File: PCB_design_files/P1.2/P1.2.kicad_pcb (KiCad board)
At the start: 2 copper layers, 127 x 127 mm, 37 parts, among them J1 -EEG_INPUT, J2 +EEG_INPUT, J3 +3.3V, J4 GND, J5 -3V3, J6 EEG_INPUT, J7 STAGE_1_OUT, J8 STAGE_2_OUT, J9 STAGE_3_OUT, U1 INA819, U2 TPS61094, U3 TLV9102, U4 TC1044

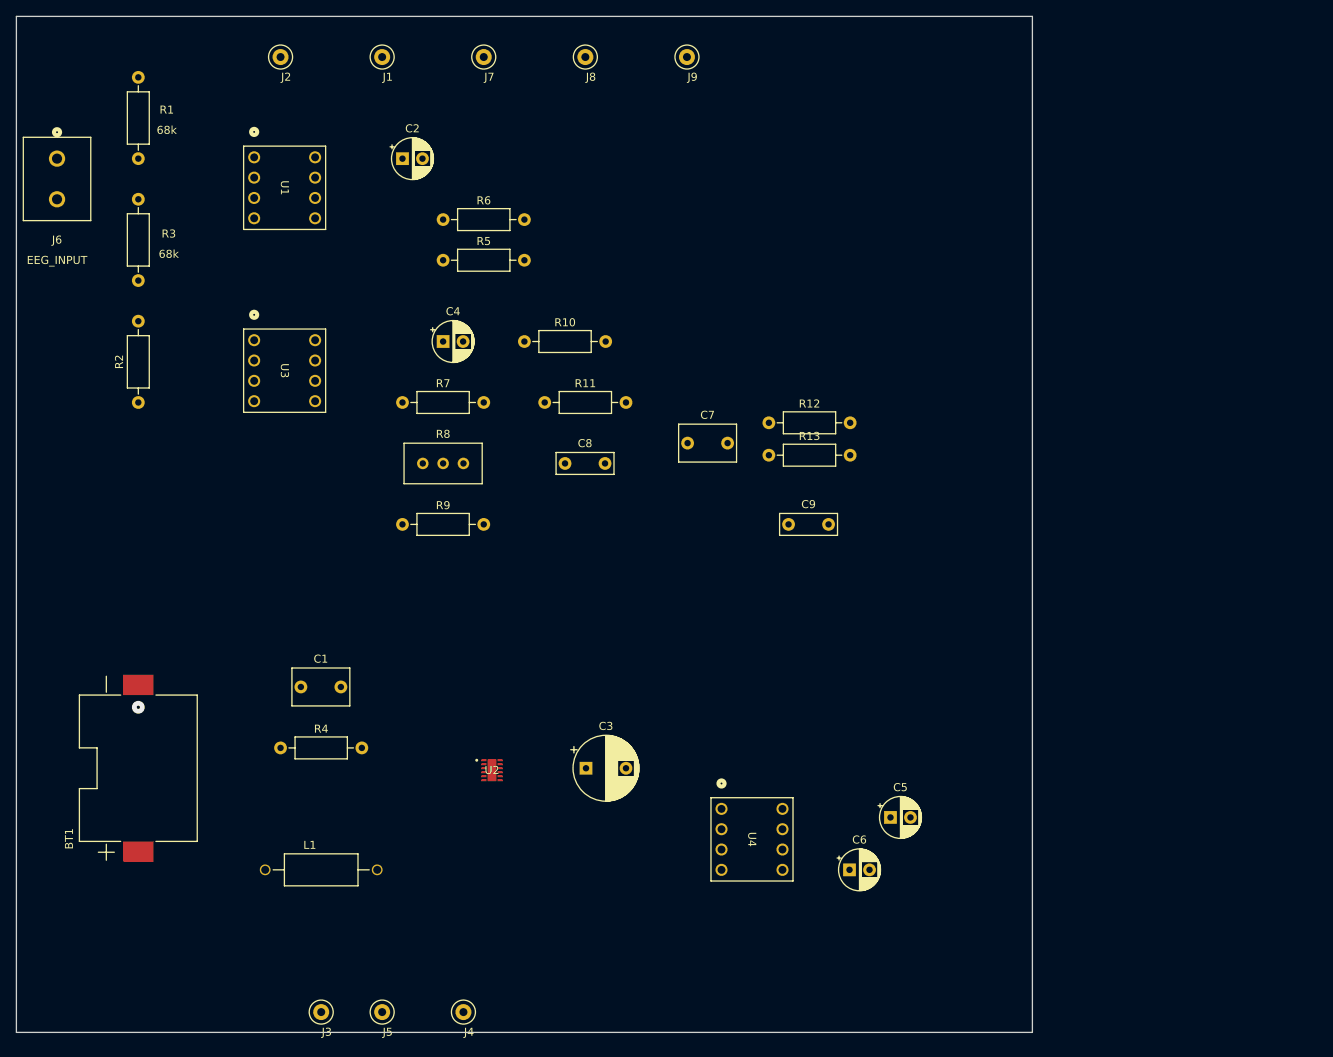
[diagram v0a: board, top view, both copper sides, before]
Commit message: Created PCB Layout
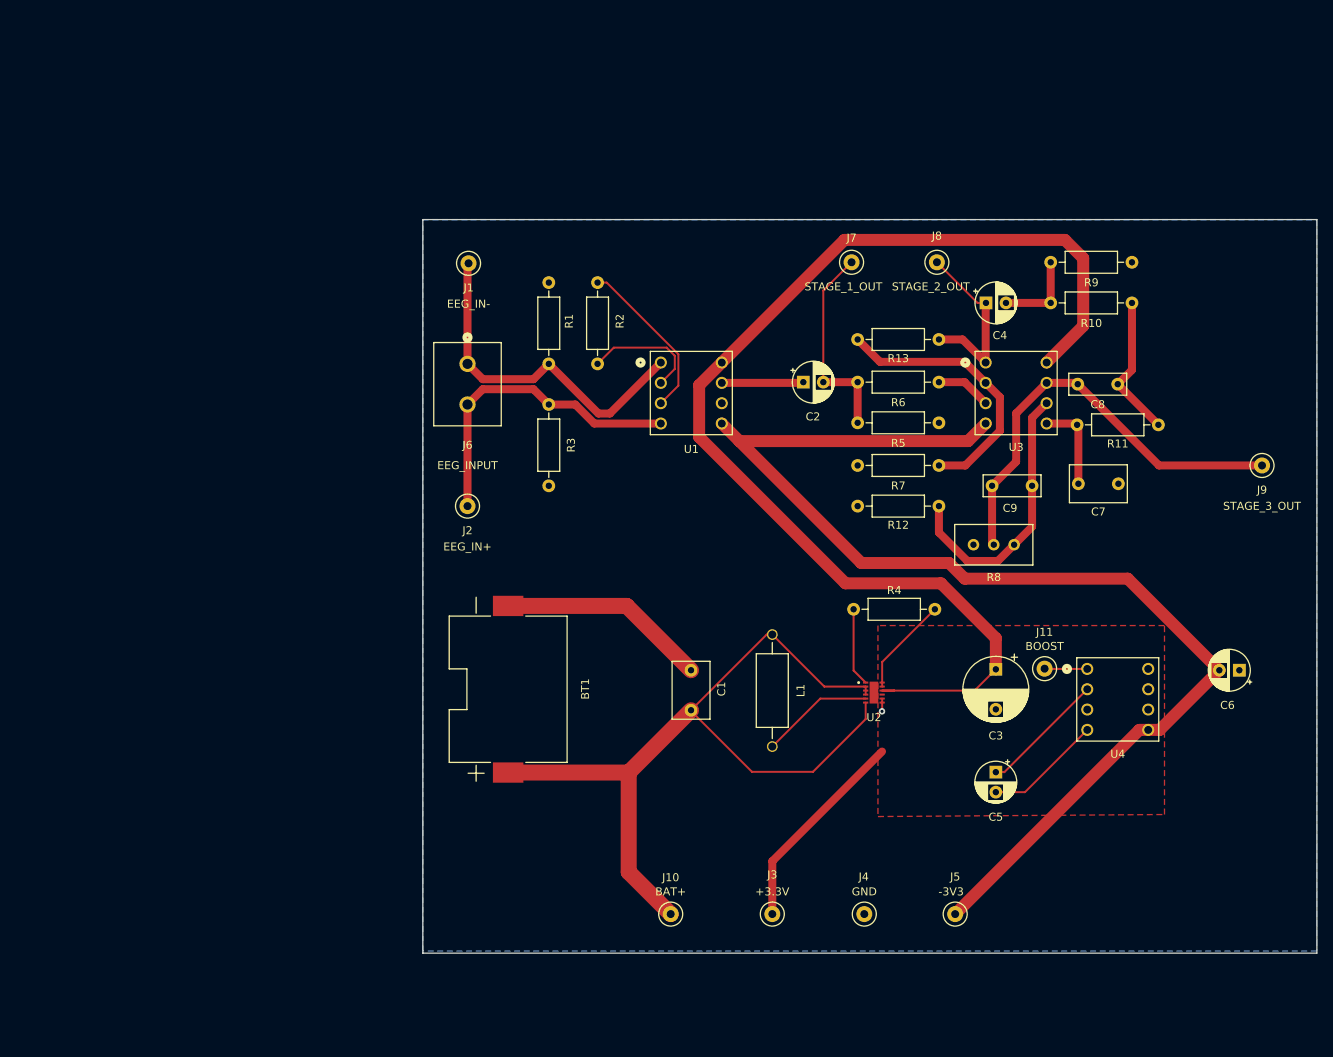
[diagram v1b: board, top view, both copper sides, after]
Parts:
- added J10: BAT+, TestPoint:TestPoint_Loop_D2.50mm_Drill1.0mm, F.Cu at (107.2, 137.6)
- added J11: BOOST, TestPoint:TestPoint_Loop_D2.50mm_Drill1.0mm, F.Cu at (153.9, 106.9)
- J1: value -EEG_INPUT -> EEG_IN-
- J2: value +EEG_INPUT -> EEG_IN+
- R13: value 50k -> 100k
- U4: value TC1044 -> TC1044S
- moved U3 91.5 mm to (146.6, 68.7), turned to 0 degrees
- moved J9 88.2 mm to (181.1, 81.5)
- moved R9 87.4 mm to (154.7, 56.1)
- moved R11 76.8 mm to (168.1, 76.5), turned to 180 degrees
- moved R4 73.7 mm to (130.0, 99.5)
- moved J5 72.7 mm to (142.7, 137.6)
- moved R8 69.6 mm to (150.1, 91.4)
- moved C4 68.0 mm to (146.6, 61.2)
- moved R10 66.0 mm to (154.7, 61.2)
- moved C8 64.8 mm to (158.1, 71.4)
- moved J2 60.8 mm to (81.8, 86.6)
- moved L1 60.7 mm to (119.9, 109.7), turned to -90 degrees
- moved J3 57.7 mm to (119.9, 137.6)
- moved R2 57.6 mm to (98.0, 68.8)
- moved R7 57.4 mm to (130.6, 81.5)
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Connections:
- net Net-(BT1-+) renamed BAT+
- net Net-(J1-Pin_1) renamed /EEG_IN-
- net Net-(J2-Pin_1) renamed /EEG_IN+
- net Net-(J7-Pin_1) renamed STAGE_1_OUT
- C4 pad 1: Net-(J8-Pin_1) -> STAGE_2_OUT
- J8 pad 1: Net-(J8-Pin_1) -> STAGE_2_OUT
- R13 pad 1: Conditioned_EEG -> STAGE_2_OUT
- R13 pad 2: Net-(U3-IN2-) -> Net-(U3-IN1-)
- R8 pad 1: +3.3V -> Net-(U3-IN2-)
- R8 pad 2: Net-(U3-IN1-) -> Conditioned_EEG
- U3 pad 1: Net-(J8-Pin_1) -> STAGE_2_OUT
- U4 pad 1: GND -> Net-(J11-Pin_1)
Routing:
- net +3.3V: track 0.00 -> 172.1 mm
- net -3V3: track 0.00 -> 152.3 mm
- net BAT+: track 0.00 -> 105.3 mm
- net Conditioned_EEG: track 0.00 -> 54.3 mm
- net /EEG_IN-: track 0.00 -> 43.8 mm
- net GND: track 0.00 -> 40.6 mm, vias 0 -> 1
- net /EEG_IN+: track 0.00 -> 39.4 mm
- net Net-(U3-IN1-): track 0.00 -> 34.4 mm
- net Net-(U3-IN2-): track 0.00 -> 34.4 mm
- net STAGE_1_OUT: track 0.00 -> 25.8 mm
- net STAGE_2_OUT: track 0.00 -> 22.7 mm
- net Net-(R2-Pad2): track 0.00 -> 20.8 mm
- net Net-(C8-Pad2): track 0.00 -> 18.1 mm
- net Net-(U4-CAP+): track 0.00 -> 15.7 mm
- net Net-(R2-Pad1): track 0.00 -> 15.0 mm
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- added copper zone on F.Cu, net +3.3V
- added copper zone on B.Cu, net GND
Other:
- board size 127 x 127 mm -> 111.8 x 91.7 mm
